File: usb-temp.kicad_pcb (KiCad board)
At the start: 4 copper layers, 20 x 17.8 mm, 11 parts, among them J1 Conn_01x02_Pin, J2 USB_MB, J3 Conn_01x05, U1 STM32F042F4Px, U2 ZLDO1117G33TA

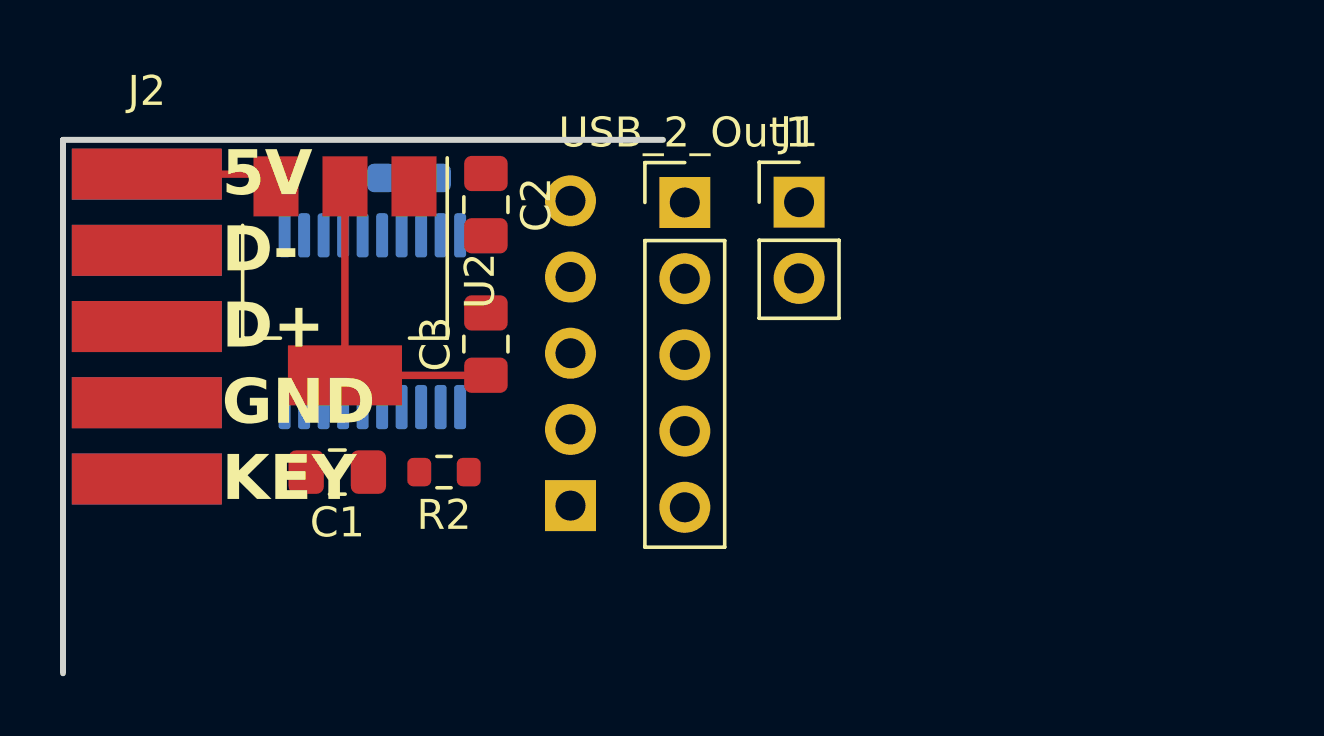
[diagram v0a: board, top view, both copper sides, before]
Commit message: First Order
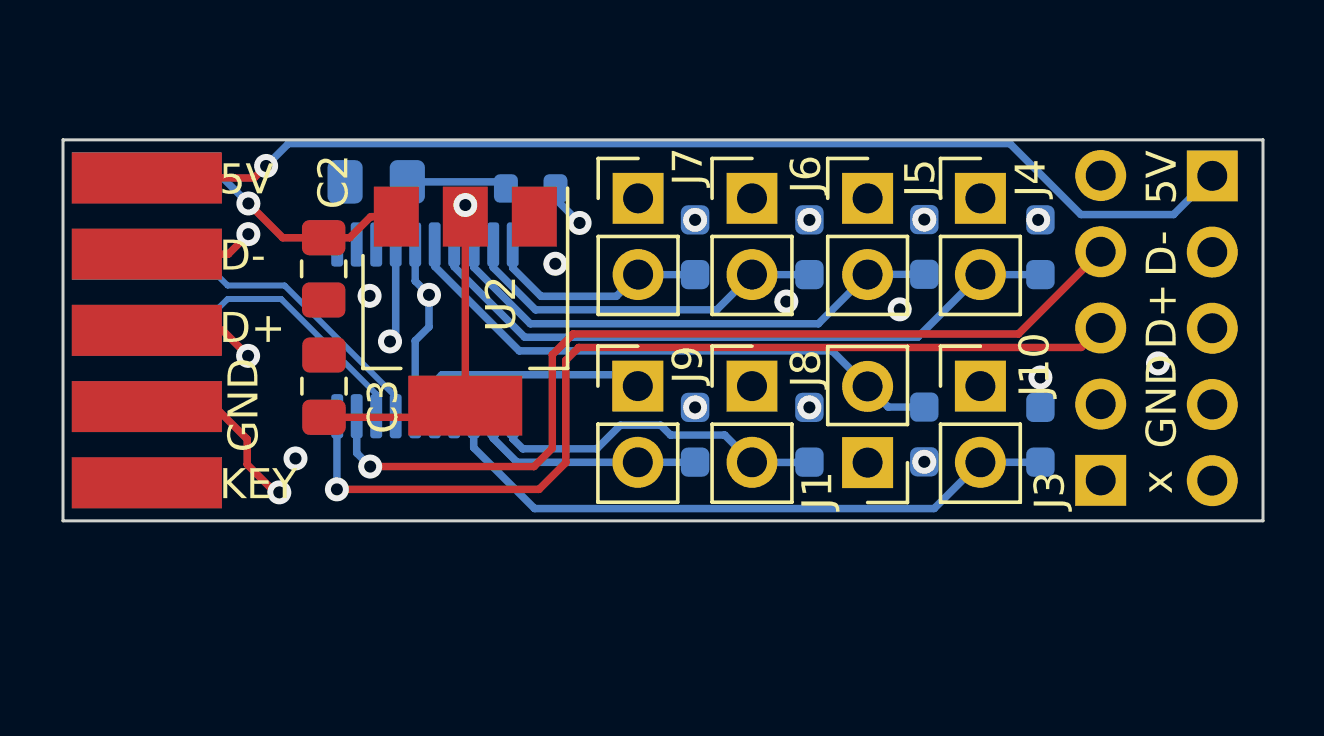
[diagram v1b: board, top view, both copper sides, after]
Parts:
- added J10: Conn_01x02_Pin, Connector_PinHeader_2.54mm:PinHeader_1x02_P2.54mm_Vertical, F.Cu at (30.6, 8.21)
- added J4: Conn_01x02_Pin, Connector_PinHeader_2.54mm:PinHeader_1x02_P2.54mm_Vertical, F.Cu at (30.6, 1.95)
- added J5: Conn_01x02_Pin, Connector_PinHeader_2.54mm:PinHeader_1x02_P2.54mm_Vertical, F.Cu at (26.8, 1.95)
- added J6: Conn_01x02_Pin, Connector_PinHeader_2.54mm:PinHeader_1x02_P2.54mm_Vertical, F.Cu at (23.0, 1.95)
- added J7: Conn_01x02_Pin, Connector_PinHeader_2.54mm:PinHeader_1x02_P2.54mm_Vertical, F.Cu at (19.2, 1.95)
- added J8: Conn_01x02_Pin, Connector_PinHeader_2.54mm:PinHeader_1x02_P2.54mm_Vertical, F.Cu at (23.0, 8.21)
- added J9: Conn_01x02_Pin, Connector_PinHeader_2.54mm:PinHeader_1x02_P2.54mm_Vertical, F.Cu at (19.2, 8.21)
- added R3: R-10k-0603, Resistor_SMD:R_0603_1608Metric_Pad0.98x0.95mm_HandSolder, B.Cu at (32.6, 3.58)
- added R4: R-10k-0603, Resistor_SMD:R_0603_1608Metric_Pad0.98x0.95mm_HandSolder, B.Cu at (28.7, 3.57)
- added R5: R-10k-0603, Resistor_SMD:R_0603_1608Metric_Pad0.98x0.95mm_HandSolder, B.Cu at (24.9, 3.58)
- added R6: R-10k-0603, Resistor_SMD:R_0603_1608Metric_Pad0.98x0.95mm_HandSolder, B.Cu at (21.1, 3.58)
- added R7: R-10k-0603, Resistor_SMD:R_0603_1608Metric_Pad0.98x0.95mm_HandSolder, B.Cu at (24.9, 9.83)
- added R8: R-10k-0603, Resistor_SMD:R_0603_1608Metric_Pad0.98x0.95mm_HandSolder, B.Cu at (21.1, 9.83)
- added R9: R-10k-0603, Resistor_SMD:R_0603_1608Metric_Pad0.98x0.95mm_HandSolder, B.Cu at (32.6, 9.83)
- C1, R2: moved to B.Cu
- J3: moved to F.Cu
- moved R1 19.2 mm to (28.7, 9.82), turned to 90 degrees
- moved J3 17.7 mm to (34.6, 11.3), turned to 180 degrees
- moved USB_2_Out1 17.6 mm to (38.3, 1.20)
- moved R2 9.89 mm to (15.6, 1.62)
- moved C1 9.76 mm to (10.4, 1.40)
- moved J1 8.98 mm to (26.8, 10.8), turned to 180 degrees
- moved C2 5.82 mm to (8.69, 4.30)
- moved C3 5.58 mm to (8.70, 8.21)
- moved U2 4.14 mm to (13.4, 5.71)
- moved U1 1.78 mm to (12.1, 6.35)
- moved J2 0.13 mm to (2.79, 1.27)
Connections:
- net Net-(J1-Pin_2) renamed /A_Input0/A
- J2 pad 1: +5V -> Net-(J2A-VBUS)
- J2 pad 2: Net-(J2B-VBUS) -> +5V
- J2 pad 3: USB_D- -> Net-(J2A-D-)
- J2 pad 4: Net-(J2B-D-) -> USB_D-
- J2 pad 5: USB_D+ -> Net-(J2A-D+)
- J2 pad 6: Net-(J2B-D+) -> USB_D+
- J2 pad 7: GND -> Net-(J2A-GND)
- J2 pad 8: Net-(J2B-GND) -> GND
- U1 pad 10: unconnected-(U1-PA4-Pad10) -> /A_Input6/A
- U1 pad 11: unconnected-(U1-PA5-Pad11) -> /A_Input5/A
- U1 pad 12: unconnected-(U1-PA6-Pad12) -> /A_Input4/A
- U1 pad 13: unconnected-(U1-PA7-Pad13) -> /A_Input7/A
- U1 pad 7: unconnected-(U1-PA1-Pad7) -> /A_Input1/A
- U1 pad 8: unconnected-(U1-PA2-Pad8) -> /A_Input2/A
- U1 pad 9: unconnected-(U1-PA3-Pad9) -> /A_Input3/A
- USB_2_Out1 pad 1: Net-(J2B-VBUS) -> Net-(J2A-VBUS)
- USB_2_Out1 pad 2: Net-(J2B-D-) -> Net-(J2A-D-)
- USB_2_Out1 pad 3: Net-(J2B-D+) -> Net-(J2A-D+)
- USB_2_Out1 pad 4: Net-(J2B-GND) -> Net-(J2A-GND)
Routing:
- net +3V3: track 11.0 -> 81.6 mm, vias 0 -> 11
- net Net-(J2A-D+): track 0.00 -> 43.8 mm, vias 0 -> 1
- net Net-(J2A-GND): track 0.00 -> 39.7 mm, vias 0 -> 1
- net Net-(J2A-D-): track 0.00 -> 38.5 mm, vias 0 -> 1
- net RST: track 0.00 -> 38.0 mm, vias 0 -> 1
- net Net-(J2A-VBUS): track 0.00 -> 37.5 mm, vias 0 -> 1
- net SWDCLK: track 0.00 -> 32.1 mm, vias 0 -> 1
- net SWDIO: track 0.00 -> 31.0 mm, vias 0 -> 1
- net /A_Input1/A: track 0.00 -> 22.1 mm
- net /A_Input7/A: track 0.00 -> 21.4 mm
- net /A_Input0/A: track 0.00 -> 19.0 mm
- net /A_Input2/A: track 0.00 -> 17.2 mm
- net /A_Input3/A: track 0.00 -> 12.4 mm
- net /A_Input5/A: track 0.00 -> 11.6 mm
- net USB_D-: track 0.00 -> 10.9 mm
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- added copper zone on B.Cu, net GND
- added copper zone on F.Cu, net GND
- added copper zone on In1.Cu, net GND
- added copper zone on In2.Cu, net GND
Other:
- board size 20 x 17.8 mm -> 40 x 12.7 mm
- board text added: "5V"
- board text added: "D+"
- board text added: "D-"
- board text added: "GND"
- board text added: "x"
